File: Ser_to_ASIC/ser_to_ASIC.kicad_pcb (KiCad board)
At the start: 2 copper layers, 52 parts, among them J200 MOLEX-524653071, J3 CONMHF4-SMD-G-T, J6 MOLEX-524653071, U1 ADP160AUJZ-1.2-R7, U2 ADP121-AUJZ12R7, U3 10M02DCV36I7G, U4 DS90UB913ATRTVJQ1, U5 TC2015-1.8VCTTR, U6 LT1761ES5-3.3-TRPBF, X1 EG-2102CA 100.0000M-PHPAL3

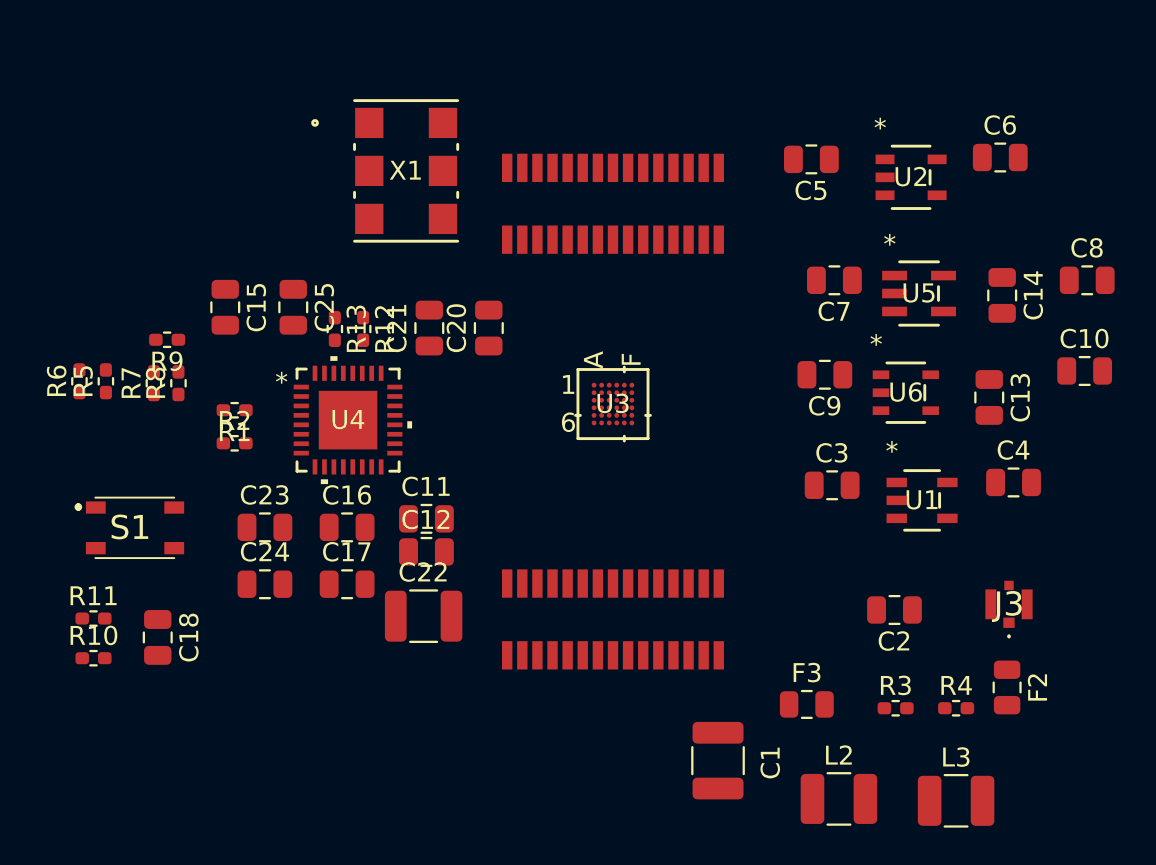
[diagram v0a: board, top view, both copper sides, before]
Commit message: actualitzacio
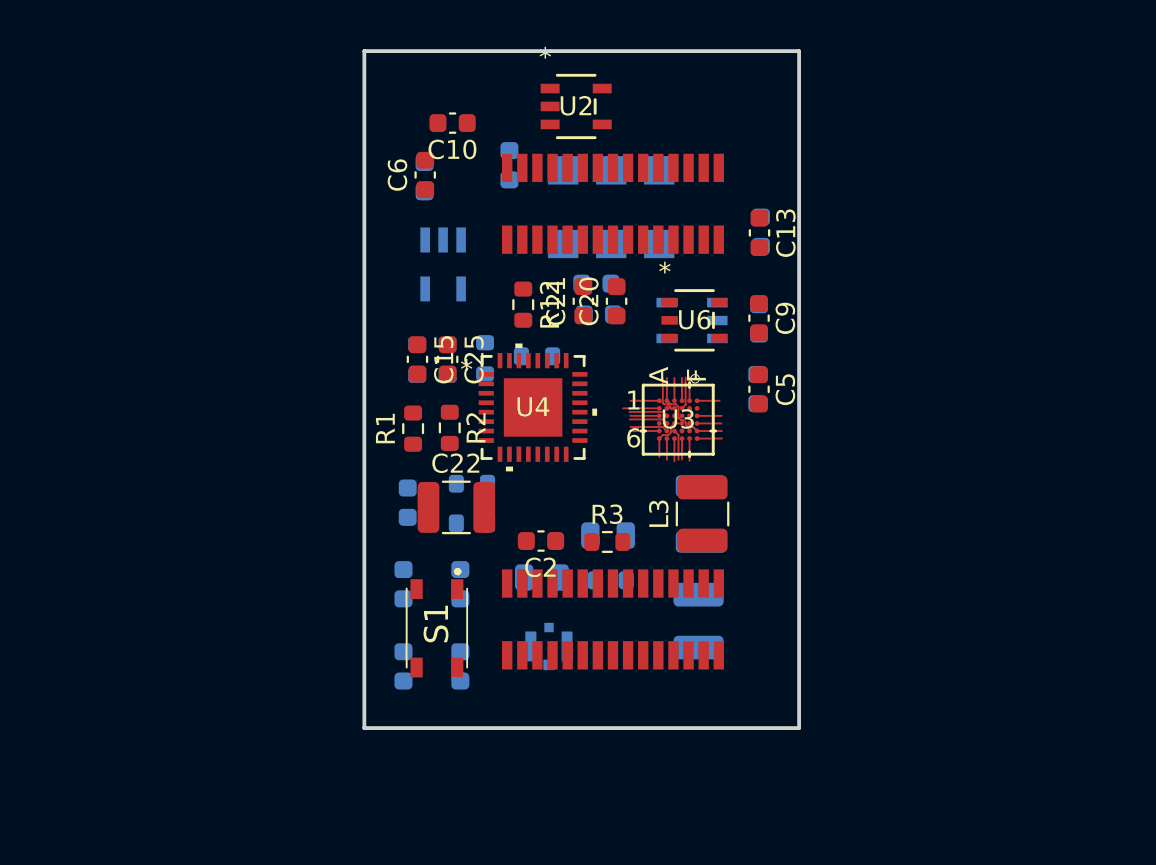
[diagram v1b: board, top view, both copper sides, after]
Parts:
- C1, F2, F3, J3, L2, U1, U5, X1: moved to B.Cu
- C10, C13, C15, C2, C20, C21, C25, C5, C6, C9: footprint Capacitor_SMD:C_0805_2012Metric -> Capacitor_SMD:C_0603_1608Metric
- C11, C12, C14, C16, C17, C18, C23, C24, C3, C4, C7, C8: footprint Capacitor_SMD:C_0805_2012Metric -> Capacitor_SMD:C_0603_1608Metric; moved to B.Cu
- R1, R12, R2, R3: footprint Resistor_SMD:R_0402_1005Metric_Pad0.72x0.64mm_HandSolder -> Resistor_SMD:R_0603_1608Metric
- R10, R11, R13, R4, R5, R6, R7, R8, R9: footprint Resistor_SMD:R_0402_1005Metric_Pad0.72x0.64mm_HandSolder -> Resistor_SMD:R_0603_1608Metric; moved to B.Cu
- moved C10 35.9 mm to (145.8, 73.2), turned to 180 degrees
- moved C6 30.5 mm to (144.4, 76.0), turned to 90 degrees
- moved C14 27.0 mm to (148.8, 75.5), turned to 90 degrees
- moved F2 25.3 mm to (150.5, 97.3), turned to 0 degrees
- moved U5 25.2 mm to (145.3, 80.7), turned to -90 degrees
- moved R6 24.6 mm to (150.7, 88.2)
- moved J3 24.5 mm to (150.9, 100.9), turned to 180 degrees
- moved C7 22.4 mm to (144.3, 76.1), turned to 90 degrees
- moved R5 21.8 mm to (149.3, 88.2)
- moved R10 21.3 mm to (146.8, 94.4), turned to 180 degrees
- moved R11 21.3 mm to (146.8, 92.3), turned to 180 degrees
- moved L3 20.3 mm to (159.0, 93.9), turned to 90 degrees
- moved R4 19.5 mm to (154.2, 97.4), turned to 180 degrees
- moved C2 19.1 mm to (150.5, 95.3)
- moved C8 18.4 mm to (161.9, 87.3), turned to -90 degrees
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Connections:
- R7 pad 1: Net-(U4-SDA) -> /SDA_SER
- R8 pad 1: Net-(U4-SCL) -> /SCL_SER
- U3 pad A1: unconnected-(U3-VCCA3-PadA1) -> +3.3V
- U3 pad A3: /MODE_1 -> /CLK_100
- U3 pad A5: /M1_B -> /SDA_SER
- U3 pad A6: unconnected-(U3-VCCA2-PadA6) -> +3.3V
- U3 pad B2: /M0_B -> unconnected-(U3-IO-PadB2)
- U3 pad B4: /SPI_CLK -> /DAC_SDI
- U3 pad B5: /SPI_DATA -> /SCL_SER
- U3 pad B6: /\SPI_CS -> /DAC_SCK
- U3 pad C1: /DAC_SCK -> /SPI_DATA
- U3 pad C2: /DAC_SDI -> /MODE_1
- U3 pad C3: /\DAC_CS -> unconnected-(U3-IO-PadC3)
- U3 pad C4: unconnected-(U3-VCCIO1_2_8-PadC4) -> +3.3V
- U3 pad C5: /PB_0 -> /PB_1
- U3 pad C6: /PB_1 -> /\DAC_CS
- U3 pad D1: /CLK_100 -> /SPI_CLK
- U3 pad D3: /CLK_25_6 -> unconnected-(U3-IO-PadD3)
- U3 pad D4: unconnected-(U3-VCCIO3_5_6-PadD4) -> +3.3V
- U3 pad D6: unconnected-(U3-IO-PadD6) -> /M0_B
- U3 pad E1: unconnected-(U3-IO-PadE1) -> /CLK_25_6
- U3 pad E6: unconnected-(U3-IO-PadE6) -> /PB_0
- U3 pad F3: /SDA_SER -> /\SPI_CS
- U3 pad F4: /SCL_SER -> /M1_B
- U3 pad F6: GND -> G
- U4 pad 4: Net-(U4-SCL) -> /SCL_SER
- U4 pad 5: Net-(U4-SDA) -> /SDA_SER
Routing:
- net +1V2: track 0.00 -> 5.18 mm
- net G: track 0.00 -> 4.57 mm
- net +3.3V: track 0.00 -> 4.20 mm
- net /MODE_1: track 0.00 -> 2.12 mm
- net /DAC_SDI: track 0.00 -> 2.06 mm
- net /SCL_SER: track 0.00 -> 2.01 mm
- net /MODE_0: track 0.00 -> 1.91 mm
- net /CLK_51_2: track 0.00 -> 1.71 mm
- net /PB_1: track 0.00 -> 1.62 mm
- net /SDA_SER: track 0.00 -> 1.55 mm
- net /CLK_100: track 0.00 -> 1.54 mm
- net /\SPI_CS: track 0.00 -> 1.30 mm
- net /M1_B: track 0.00 -> 1.29 mm
- net /CLK_25_6: track 0.00 -> 1.27 mm, vias 0 -> 1
- net /SPI_CLK: track 0.00 -> 1.22 mm
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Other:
- board outline added: 23 x 35.8 mm

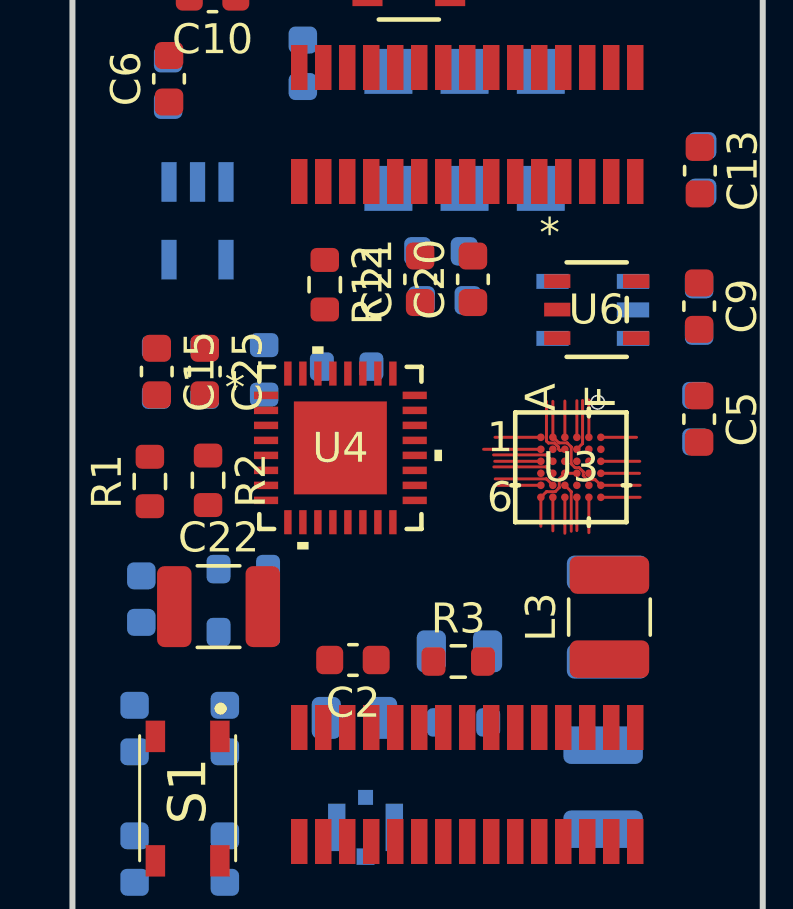
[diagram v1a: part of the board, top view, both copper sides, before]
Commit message: ACTUALITZACIO
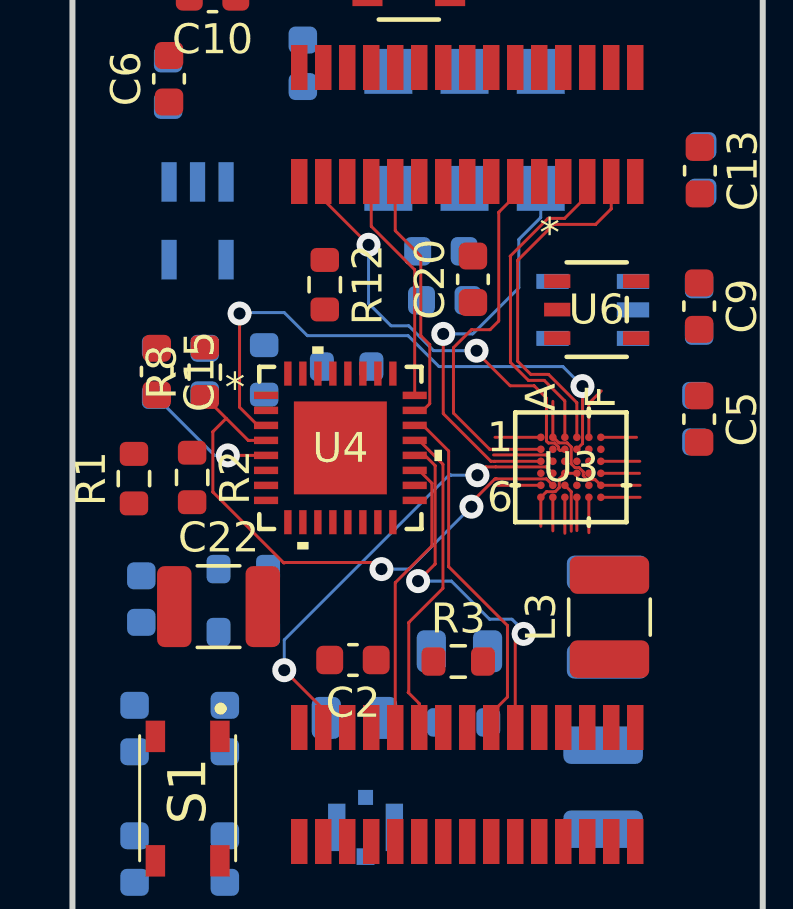
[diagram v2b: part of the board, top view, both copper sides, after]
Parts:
- removed C21: 0.1uF, Capacitor_SMD:C_0603_1608Metric
- C25: moved to B.Cu
- R8: moved to F.Cu
- moved R1 0.54 mm to (143.2, 89.3)
- moved R2 0.54 mm to (145.1, 89.3)
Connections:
- U3 pad D2: /CLK_51_2 -> /SCLK
- U3 pad E1: /CLK_25_6 -> /OSC_CLK
- U4 pad 3: /CLK_51_2 -> /SCLK
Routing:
- net /SCLK: track 0.00 -> 18.9 mm, vias 0 -> 2
- net /SCL_SER: track 2.01 -> 19.2 mm, vias 0 -> 2
- net /DAC_SDI: track 2.06 -> 15.0 mm, vias 0 -> 2
- net /SER_B1: track 0.00 -> 12.3 mm, vias 0 -> 2
- net /MODE_1: track 2.12 -> 14.2 mm, vias 0 -> 2
- net /CLK_100: track 1.54 -> 13.4 mm, vias 0 -> 1
- net /SER_B3: track 0.00 -> 11.7 mm
- net /SER_B2: track 0.00 -> 10.7 mm
- net /SPI_CLK: track 1.22 -> 11.8 mm
- net /MODE_0: track 1.91 -> 12.3 mm
- net /SPI_DATA: track 1.21 -> 11.0 mm
- net /SER_B0: track 0.00 -> 9.40 mm
- net /SER_B4: track 0.00 -> 8.48 mm
- net /SER_B5: track 0.00 -> 7.73 mm
- net /SDA_SER: track 1.55 -> 6.44 mm, vias 0 -> 1
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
